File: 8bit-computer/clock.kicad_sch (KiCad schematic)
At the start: 24 parts, among them SW1 SW_Push, SW2 SW_SPDT, U1 LM555xN, U2 LM555xN, U3 LM555xN, U4 74LS04, U5 74LS08, U6 74LS32

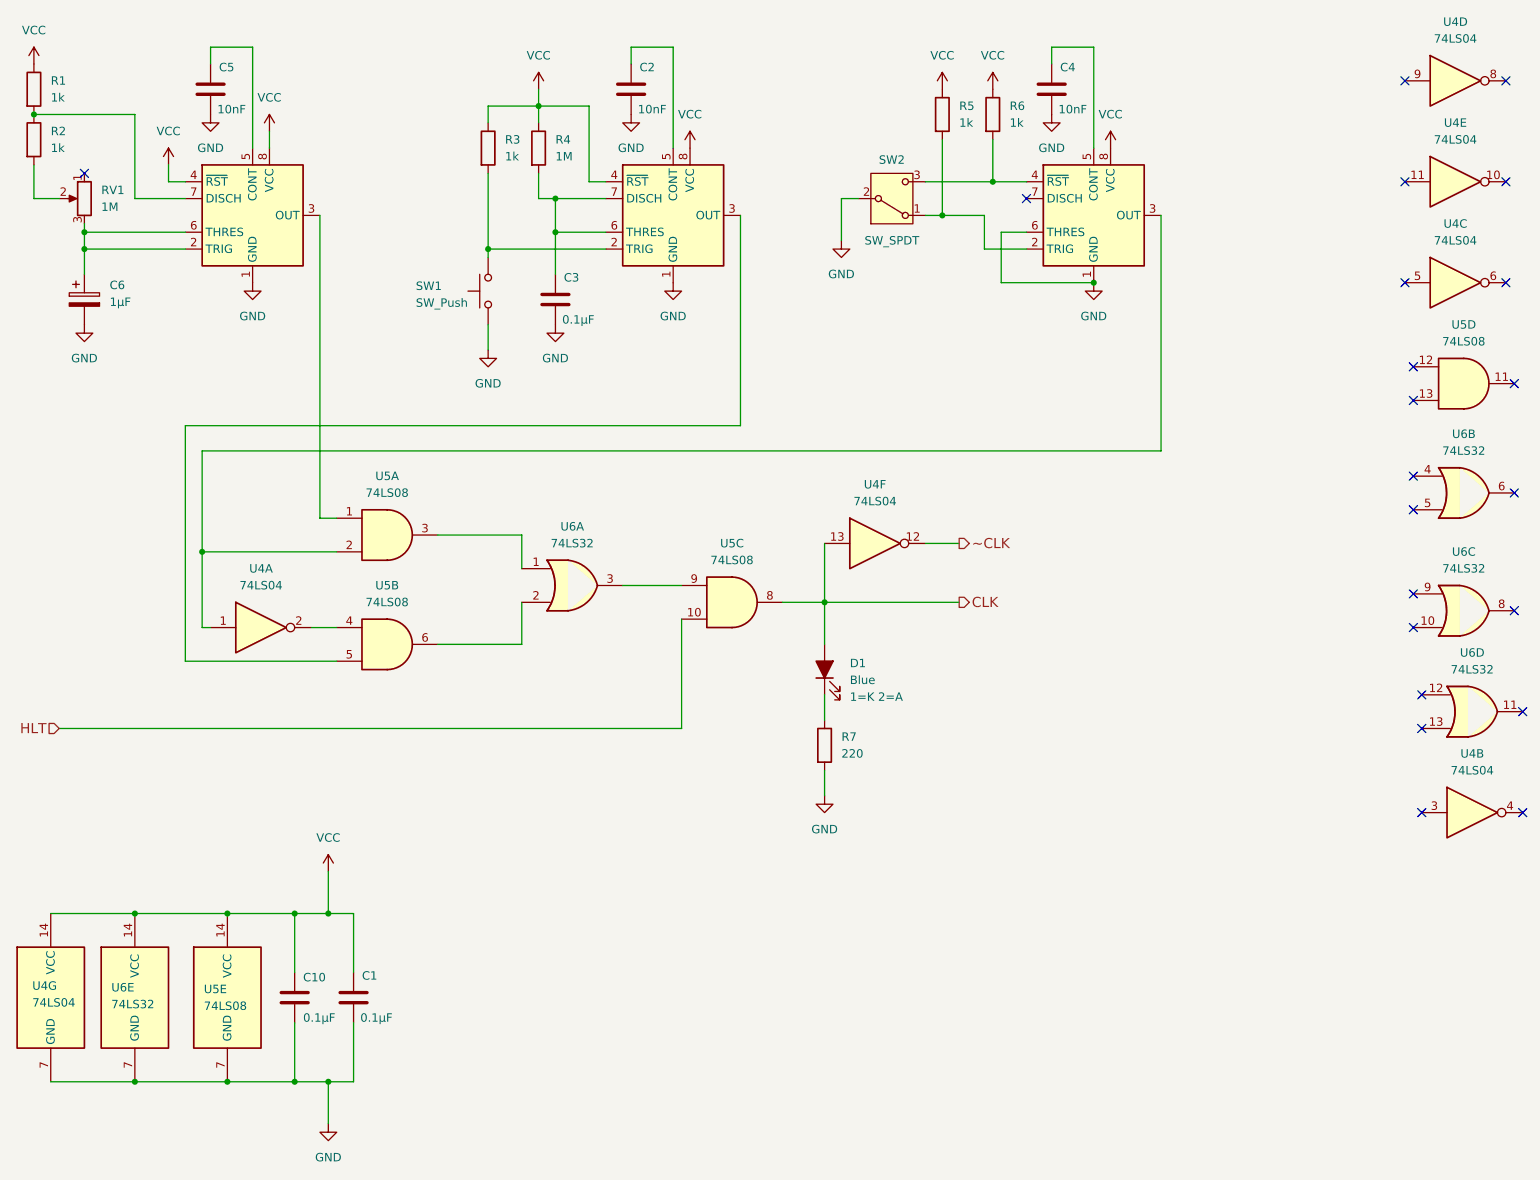
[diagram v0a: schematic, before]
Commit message: cont. 8bit schematics
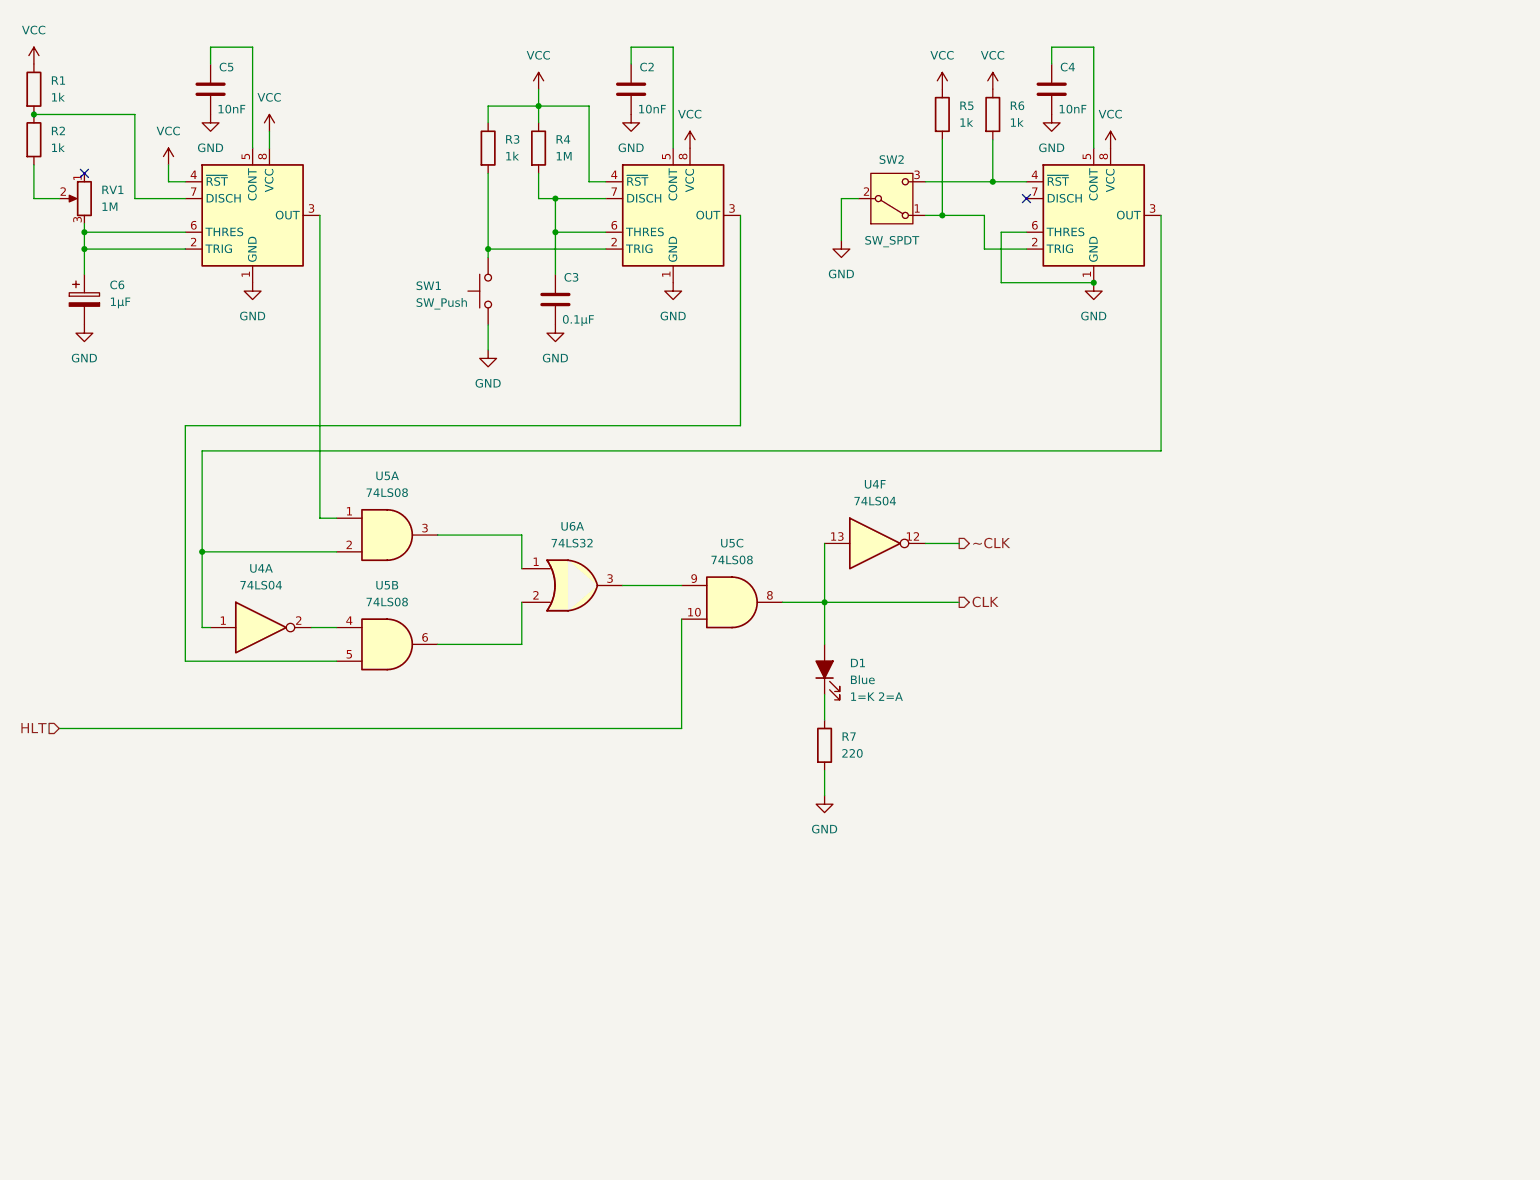
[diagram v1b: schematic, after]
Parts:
- removed C1, C10: 0.1µF, symbol Device:C
- removed unit 3 of U4
- removed unit 2 of U4
- removed unit 4 of U4
- removed unit 5 of U4
- removed unit 7 of U4
- removed unit 4 of U5
- removed unit 5 of U5
- removed unit 3 of U6
- removed unit 5 of U6
- removed unit 4 of U6
- removed unit 2 of U6
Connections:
- no-connect marks 22 -> 2
